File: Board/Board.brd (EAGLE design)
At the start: 54.2 x 85.1 mm, 68 parts, among them IC1 MEGA328, IC2 LM358D, IC4 MCP3426, IC6 MCP4921, IC7 TL431CD, Q1 IRLIZ44N, T1 BC817, U1 CJT1117-3.3-SOT223, U3 MCP9701AT-E/TT, U4 IRLML2502

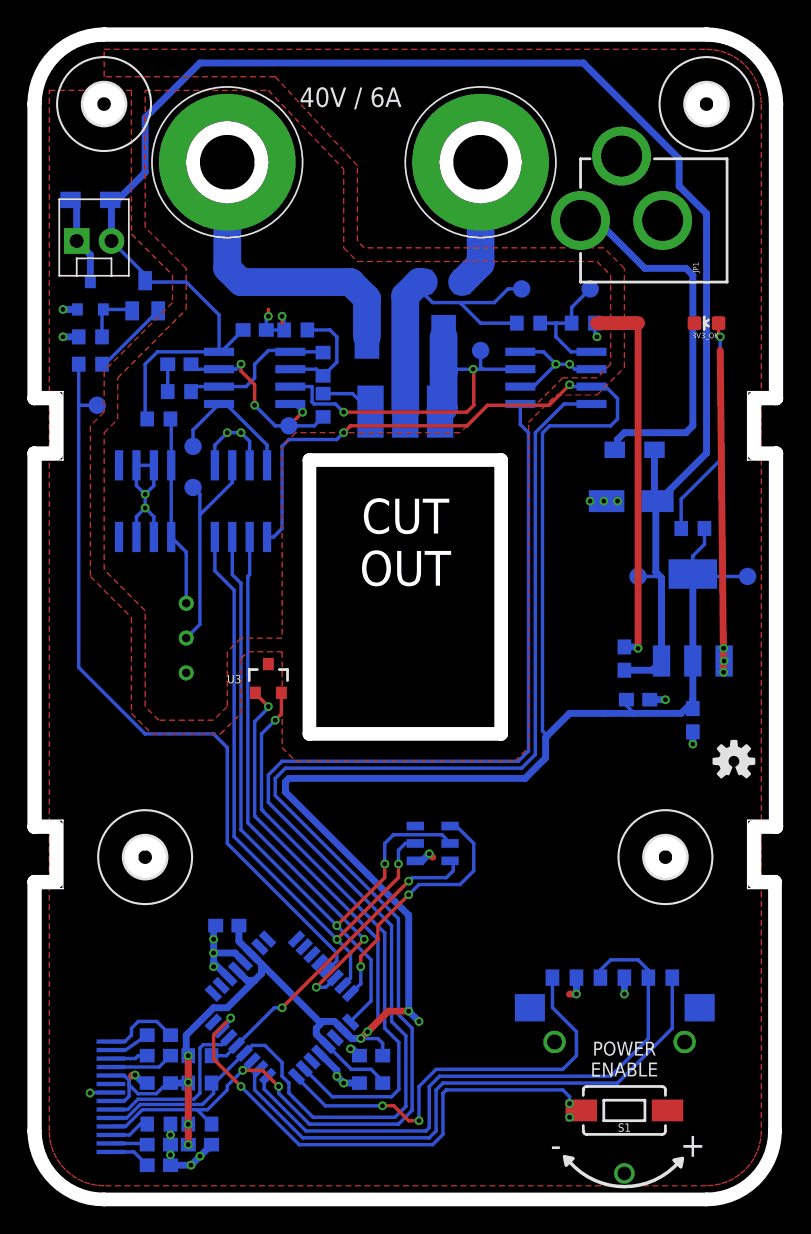
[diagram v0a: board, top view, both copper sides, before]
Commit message: added link to github repo
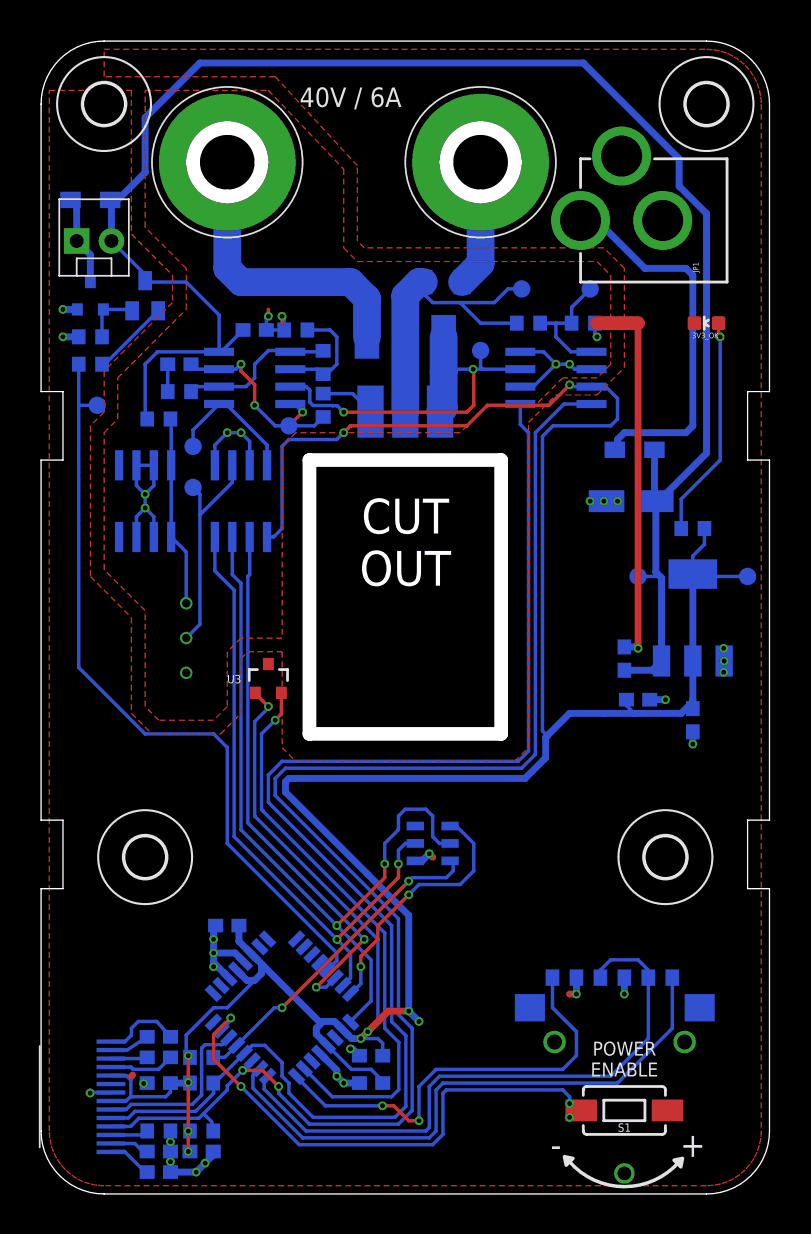
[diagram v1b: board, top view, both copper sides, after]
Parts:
- moved U$3 17.1 mm to (36.5, 20.5), flipped to the bottom
- moved U$1 15.2 mm to (31.0, 20.0)
- moved C10 0.52 mm to (11.1, 2.50)
- moved R11 0.52 mm to (11.1, 4.00)
- moved C14 0.50 mm to (8.00, 1.00)
- moved C15 0.50 mm to (8.00, 2.50)
- moved R10 0.50 mm to (8.00, 4.00)
- moved R9 0.18 mm to (11.1, 9.38)
- moved C12 0.12 mm to (8.00, 9.38)
- moved C13 0.12 mm to (8.00, 10.9)
- moved R14 0.12 mm to (11.1, 7.50)
- moved R8 0.12 mm to (20.0, 60.1)
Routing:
- net GND: track 139.2 -> 115.0 mm
- net SCK: track 53.3 -> 56.3 mm
- net +3V3: track 222.7 -> 224.3 mm
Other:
- board size 54.2 x 85.1 mm -> 53.2 x 84.2 mm
- board text added: "github.com/dangrie158/pocket-load"
